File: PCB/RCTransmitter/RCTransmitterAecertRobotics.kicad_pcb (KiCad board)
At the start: 2 copper layers, 141.6 x 100.6 mm, 41 parts, among them K1 KCD1 Power Switch

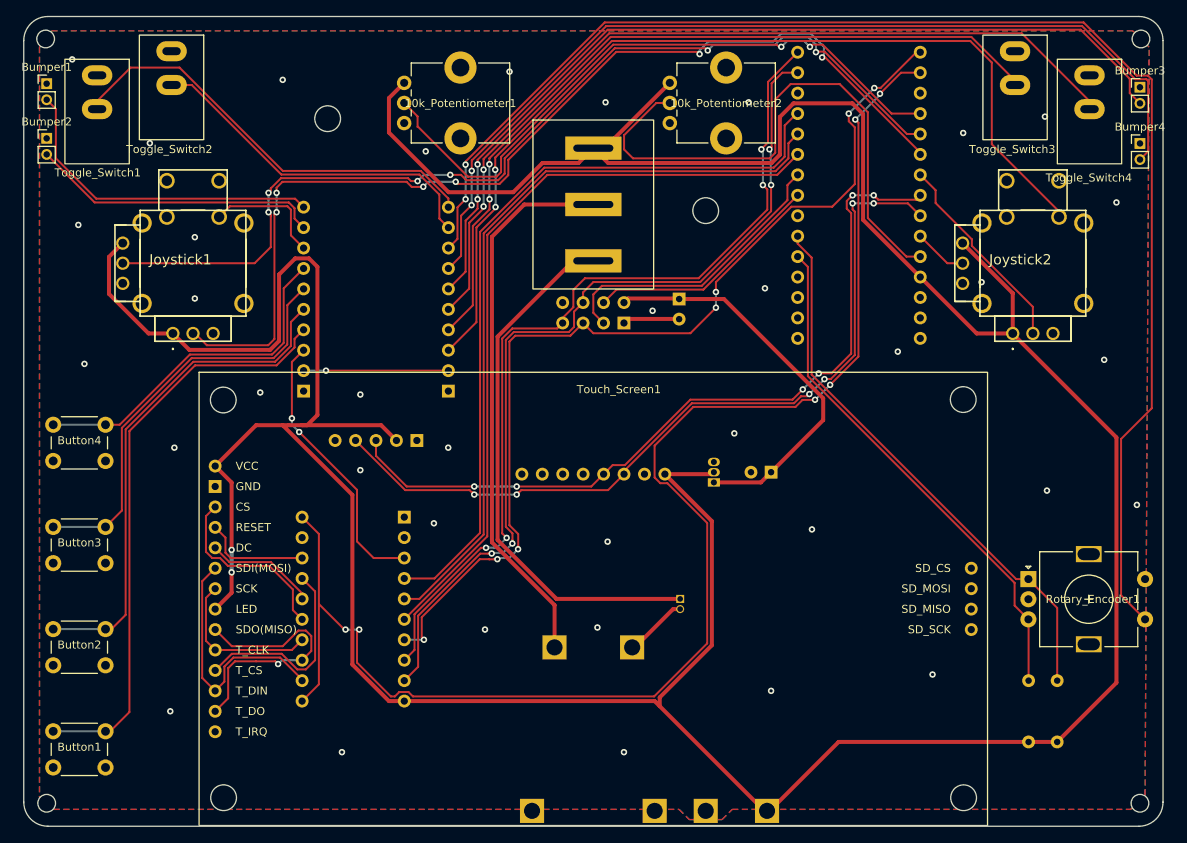
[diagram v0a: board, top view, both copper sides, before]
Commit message: nrf stuff
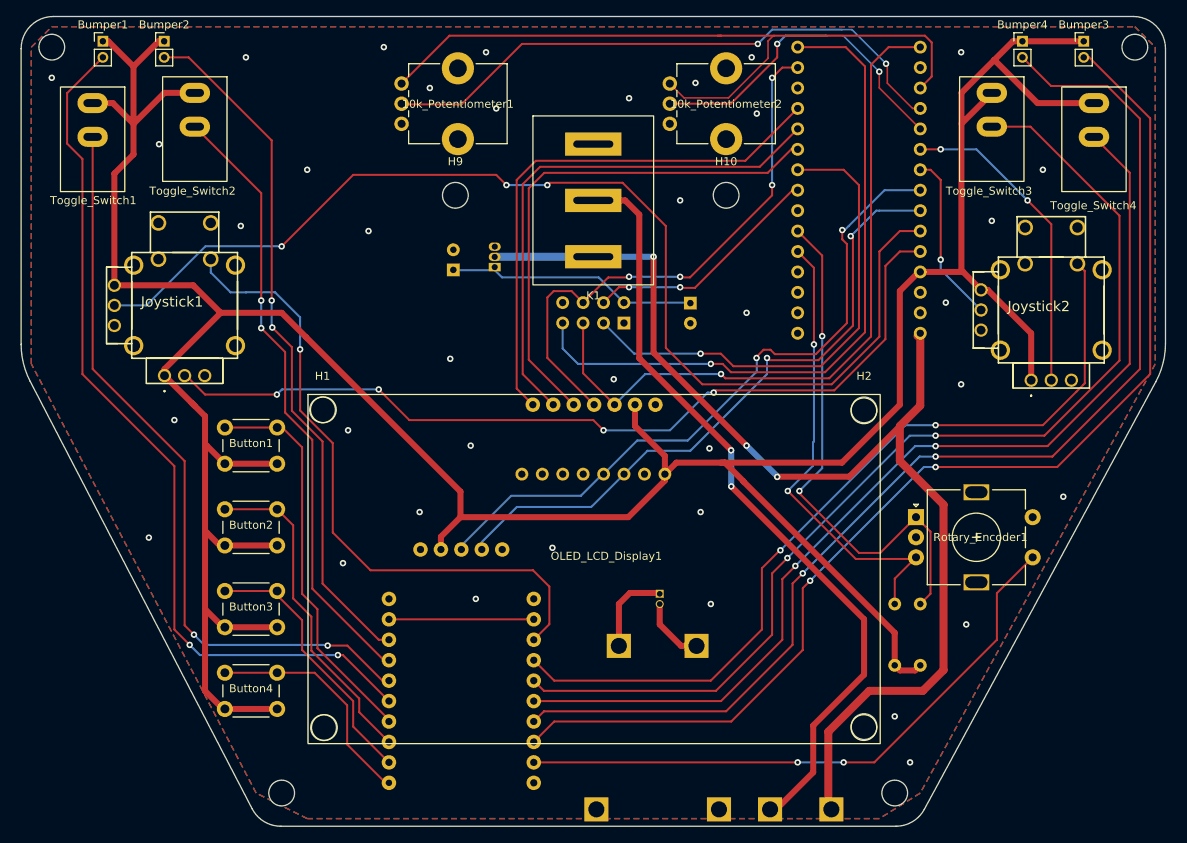
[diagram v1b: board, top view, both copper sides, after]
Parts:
- removed Level_Shifter1: TXS0108EPW, AddedFootprints:HW-221 Level Shifter
- removed Touch_Screen1: Hosyond 3.5 Inch TFT Touch Screen ILI9488, AddedFootprints:3.5 Inch Screen SPI_Module_ILI9488
- added OLED_LCD_Display1: SSD1309 2.4inch, AddedFootprints:OLED LCD Display SSD1309, F.Cu at (116.9, 90.2)
- H1, H10, H2, H9: footprint MountingHole:MountingHole_2.2mm_M2 -> MountingHole:MountingHole_3.2mm_M3
- moved H6 100.7 mm to (219.7, 47.0)
- moved H10 91.4 mm to (168.9, 65.4)
- moved H9 91.1 mm to (135.3, 65.4)
- moved H8 83.8 mm to (85.1, 47.0)
- moved IO_Extender1 75.3 mm to (125.5, 139.9), turned to 0 degrees
- moved H1 57.5 mm to (118.7, 92.1)
- moved H2 57.5 mm to (186.1, 92.1)
- moved C10uf_3 46.8 mm to (135.0, 74.7), turned to 90 degrees
- moved Button1 43.4 mm to (113.1, 98.8)
- moved H5 42.6 mm to (118.9, 131.6)
- moved H7 42.5 mm to (186.1, 131.4)
- moved 3.3V_Regulator1 38.2 mm to (140.1, 74.3)
- moved Button4 37.5 mm to (113.1, 129.2)
- moved Button2 26.0 mm to (113.1, 108.9)
- moved Button3 22.8 mm to (113.1, 119.1)
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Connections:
- 10k_Potentiometer1 pad 3: /5v -> /REF
- 10k_Potentiometer2 pad 3: /5v -> /REF
- 3.3V_Regulator1 pad 2: /5v -> /Vin
- Arduino_Nano_V3 pad 10: /TFT CS -> /Screen RES
- Arduino_Nano_V3 pad 11: /TFT DC -> /Screen DC
- Arduino_Nano_V3 pad 12: /Touch Screen CS -> /Screen CS
- Arduino_Nano_V3 pad 18: unconnected-(Arduino_Nano_V3-AREF-Pad18) -> /REF
- Arduino_Nano_V3 pad 20: /Joy Left Y -> /Pot Right
- Arduino_Nano_V3 pad 21: /Joy Left X -> /Joy Right X
- Arduino_Nano_V3 pad 22: /Joy Right X -> /Joy Right Y
- Arduino_Nano_V3 pad 25: /Joy Right Y -> /Joy Left Y
- Arduino_Nano_V3 pad 26: /Pot Right -> /Joy Left X
- Arduino_Nano_V3 pad 30: unconnected-(Arduino_Nano_V3-VIN-Pad30) -> /Vin
- Battery_Charger1 pad 1: /5v -> /Vin
- Battery_Charger1 pad 2: GND -> Net-(Battery_Charger1-VOUT-)
- Bumper1 pad 1: GND -> /5v
- Bumper2 pad 1: GND -> /5v
- Bumper3 pad 1: GND -> /5v
- Bumper4 pad 1: GND -> /5v
- Button1 pad 1: GND -> /5v
- Button2 pad 1: GND -> /5v
- Button3 pad 1: GND -> /5v
- Button4 pad 1: GND -> /5v
- Gyroscope1 pad 3: /SCL (A5) -> /SCL
- Gyroscope1 pad 4: /SDA (A4) -> /SDA
- IO_Extender1 pad 0: /TFT Reset -> /Joy Left Button
- IO_Extender1 pad 1: /Button A -> /Joy Right Button
- IO_Extender1 pad 10: /Toggle A -> /Button D
- IO_Extender1 pad 11: /Toggle B -> /Button C
- IO_Extender1 pad 12: /Rotary Encoder Switch -> /Button B
- IO_Extender1 pad 13: /Right Bumper B -> /Button A
- IO_Extender1 pad 14: /Right Bumper A -> /Left Bumper A
- IO_Extender1 pad 15: /Toggle D -> /Toggle A
- IO_Extender1 pad 16: /Toggle C -> /Toggle B
- IO_Extender1 pad 17: /Joy Right Button -> /Left Bumper B
- IO_Extender1 pad 2: /Button B -> /Toggle C
- IO_Extender1 pad 21: /SDA (A4) -> /SDA
- IO_Extender1 pad 22: /SCL (A5) -> /SCL
- IO_Extender1 pad 3: /Button C -> /Toggle D
- IO_Extender1 pad 4: /Button D -> /Right Bumper B
- IO_Extender1 pad 5: /Joy Left Button -> /Right Bumper A
- IO_Extender1 pad 6: /Left Bumper B -> /Rotary Encoder Switch
- IO_Extender1 pad 7: /Left Bumper A -> unconnected-(IO_Extender1-P07-Pad7)
- JST_Connector1 pad 1: Net-(JST_Connector1-Pin_1) -> Net-(Battery_Charger1-BAT+)
- K1 pad 1: /5v -> GND
- K1 pad 2: Net-(Battery_Charger1-BAT+) -> Net-(Battery_Charger1-VOUT-)
- K1 pad 3: Net-(JST_Connector1-Pin_1) -> /Vin
- Toggle_Switch1 pad 1: GND -> /5v
- Toggle_Switch2 pad 1: GND -> /5v
- Toggle_Switch3 pad 1: GND -> /5v
- Toggle_Switch4 pad 1: GND -> /5v
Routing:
- net /3.3v: track 182.1 -> 0.00 mm, vias 6 -> 0
- net /Vin: track 0.00 -> 144.2 mm, vias 0 -> 3
- net /Rotary Encoder Switch: track 176.9 -> 76.0 mm
- net /SCL (A5): track 100.3 -> 0.00 mm, vias 6 -> 0
- net /SDA (A4): track 98.5 -> 0.00 mm, vias 6 -> 0
- net Net-(Battery_Charger1-VOUT-): track 0.00 -> 97.2 mm, vias 0 -> 2
- net /Touch Screen CS: track 97.0 -> 0.00 mm
- net /TFT DC: track 95.9 -> 0.00 mm
- net /TFT CS: track 94.8 -> 0.00 mm
- net /REF: track 0.00 -> 93.5 mm
- net /SDA: track 0.00 -> 85.0 mm, vias 0 -> 2
- net /SCL: track 0.00 -> 80.8 mm, vias 0 -> 2
- net /5v: track 485.5 -> 416.8 mm, vias 2 -> 0
- net /Left Bumper A: track 41.1 -> 108.8 mm, vias 0 -> 2
- net /Screen CS: track 0.00 -> 67.4 mm
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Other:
- board size 141.6 x 100.6 mm -> 142.2 x 100.6 mm
